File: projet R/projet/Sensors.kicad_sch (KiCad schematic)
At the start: 10 parts, among them J4 BORDER, J6 LIDAR, J7 BORDER, U4 ADXL343

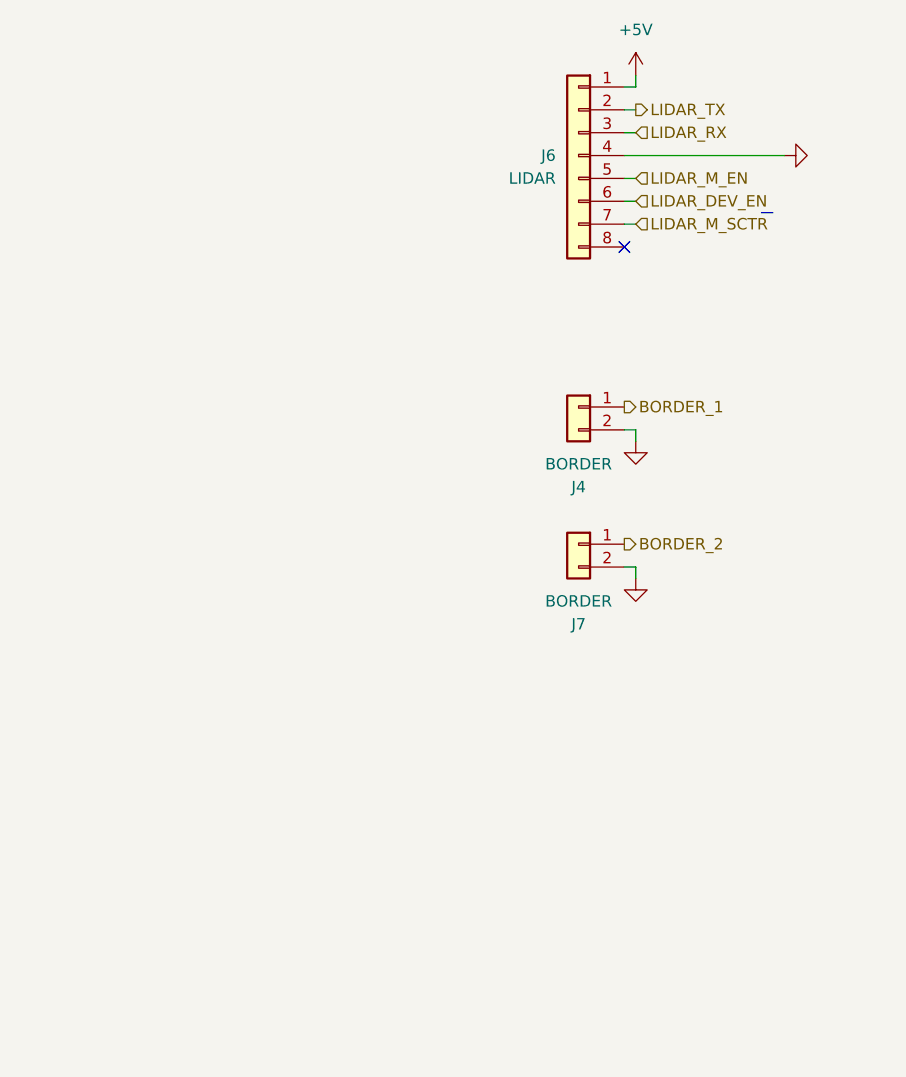
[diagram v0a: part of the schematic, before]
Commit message: Update KiCad schematics
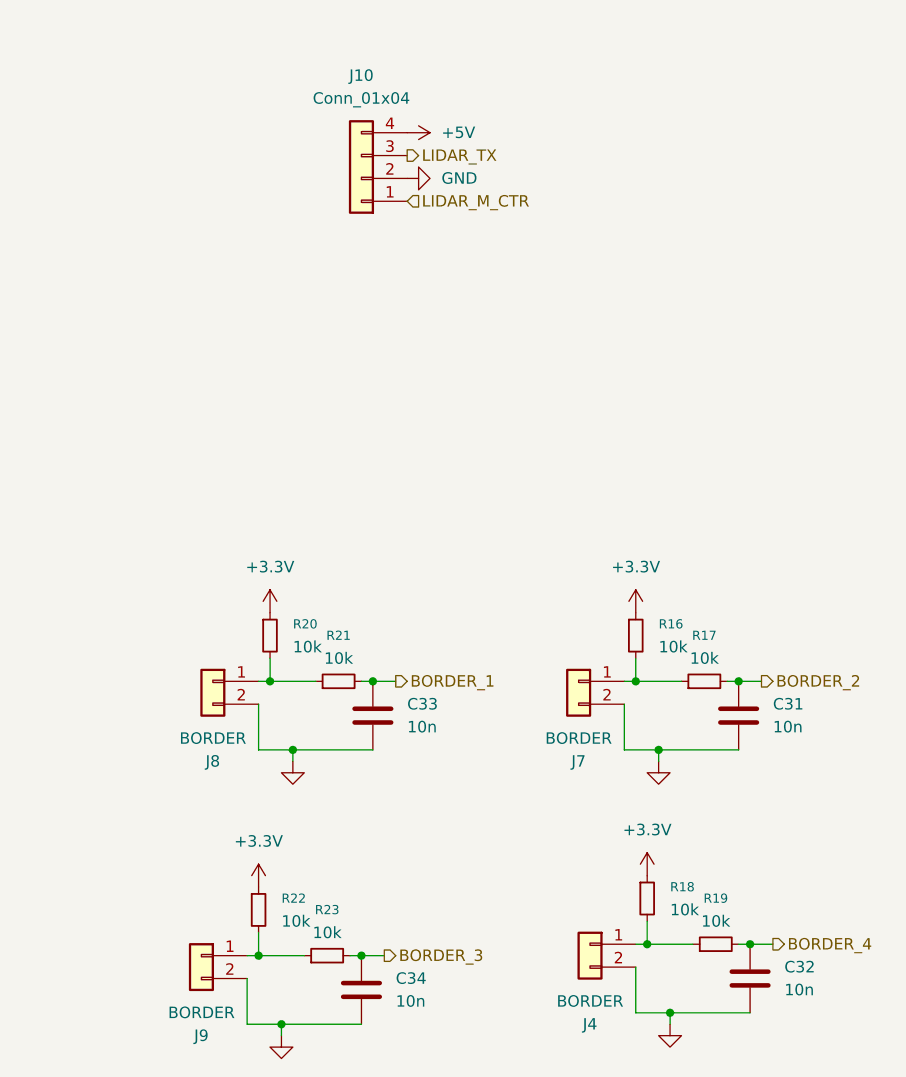
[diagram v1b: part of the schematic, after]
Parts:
- removed J6: LIDAR, Connector_JST:JST_XH_S8B-XH-A_1x08_P2.50mm_Horizontal, symbol Connector_Generic:Conn_01x08
- added C31, C32, C33, C34: 10n, symbol Device:C
- added J10: Conn_01x04, symbol Connector_Generic:Conn_01x04
- added J8, J9: BORDER, Connector_JST:JST_XH_S2B-XH-A_1x02_P2.50mm_Horizontal, symbol Connector_Generic:Conn_01x02
- added R16, R17, R18, R19, R20, R21, R22, R23: 10k, symbol Device:R_Small
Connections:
- net +3.3V: now also R16.1, R18.1, R20.1, R22.1
- net +5V: now also J10.4 (Pin_4)
- net BORDER_1: now also C33.1, R21.2; no longer J4.1 (Pin_1)
- net BORDER_2: now also C31.1, R17.2; no longer J7.1 (Pin_1)
- net GND: now also C31.2, C32.2, C33.2, C34.2, J10.2 (Pin_2), J8.2 (Pin_2), J9.2 (Pin_2)
- net LIDAR_TX: now also J10.3 (Pin_3)
- new net: J7.1 (Pin_1), R16.2, R17.1
- new net: J9.1 (Pin_1), R22.2, R23.1
- new net: J4.1 (Pin_1), R18.2, R19.1
- new net: J8.1 (Pin_1), R20.2, R21.1
- new net BORDER_3: C34.1, R23.2
- new net BORDER_4: C32.1, R19.2
- new net LIDAR_M_CTR: J10.1 (Pin_1)
- no-connect marks 3 -> 2
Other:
- moved on the sheet: J7
